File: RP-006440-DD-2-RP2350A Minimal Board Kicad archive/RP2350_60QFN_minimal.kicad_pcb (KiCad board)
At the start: 2 copper layers, 52 x 51 mm, 45 parts, among them J1 USB_C_Receptacle_USB2.0_16P, J2 Conn_02x18_Odd_Even, J3 Conn_02x18_Odd_Even, J4 SM03B-SRSS-TB, SW1 SW_Push, SW2 SW_Push, U1 RP2350_60QFN, U2 NCP1117-3.3_SOT223, U3 W25Q128JVS, Y1 ABM8-272-T3

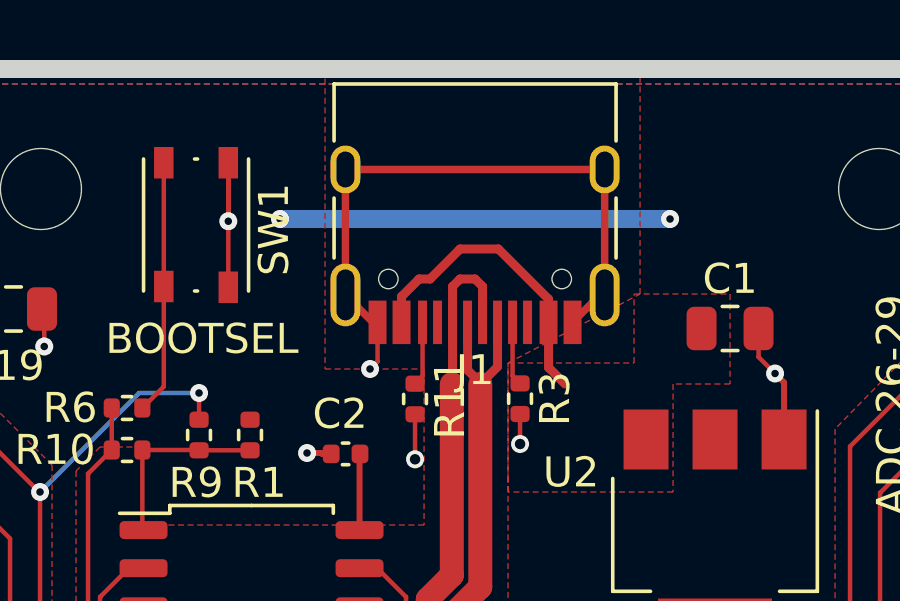
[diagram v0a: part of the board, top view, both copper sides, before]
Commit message: Schematic text
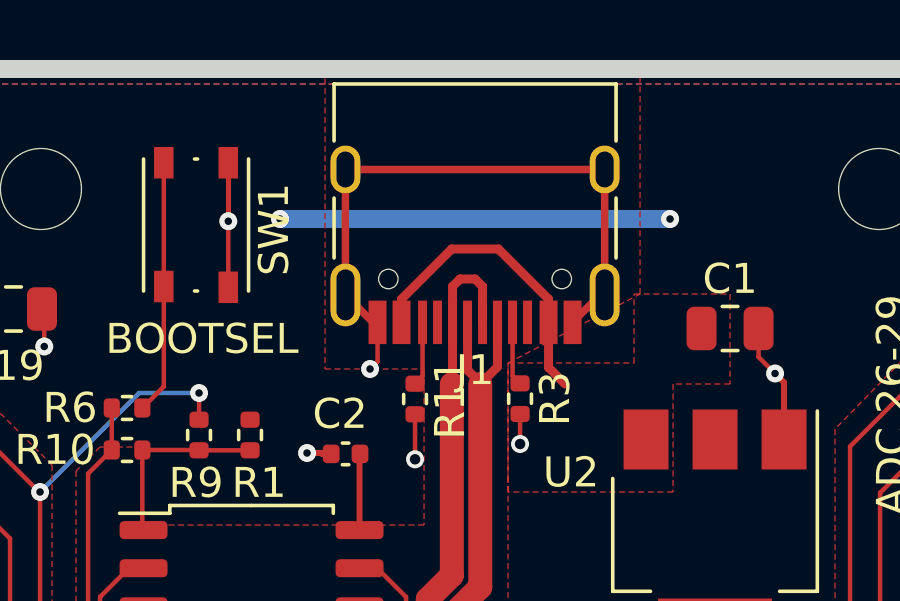
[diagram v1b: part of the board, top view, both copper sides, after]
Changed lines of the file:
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@@
 		(tags "usb usb-c 2.0 pd")
 		(property "Reference" "J1"
-			(at 0 -5.645 360)
+			(at 0 -5.645 0)
 			(layer "F.SilkS")
 			(effects
@@
 		)
 		(property "Value" "USB_C_Receptacle_USB2.0_16P"
-			(at 0 5.1 360)
+			(at 0 5.1 0)
 			(layer "F.Fab")
 			(effects
@@
 		)
 		(fp_text user "${REFERENCE}"
-			(at 0 0 360)
+			(at 0 0 0)
 			(layer "F.Fab")
 			(effects
@@
 	)
 	(segment
-		(start 100 76)
-		(end 101.28 76)
+		(start 102.95 79.95)
+		(end 103.5 80.5)
 		(width 0.3)
 		(layer "F.Cu")
@@
 	)
 	(segment
-		(start 98.05 78.445)
-		(end 98.05 77.585305)
-		(width 0.3)
-		(layer "F.Cu")
-		(net 2)
-	)
-	(segment
-		(start 102.95 79.95)
-		(end 103.5 80.5)
-		(width 0.3)
-		(layer "F.Cu")
-		(net 2)
-	)
-	(segment
-		(start 99 77)
-		(end 100 76)
+		(start 99.72 76)
+		(end 101.28 76)
 		(width 0.3)
 		(layer "F.Cu")
@@
 	)
 	(segment
-		(start 98.635305 77)
-		(end 99 77)
+		(start 102.95 78.445)
+		(end 102.95 79.95)
 		(width 0.3)
 		(layer "F.Cu")
@@
 	)
 	(segment
-		(start 102.95 78.445)
-		(end 102.95 79.95)
+		(start 101.28 76)
+		(end 102.95 77.67)
 		(width 0.3)
 		(layer "F.Cu")
@@
 	)
 	(segment
-		(start 101.28 76)
-		(end 102.95 77.67)
+		(start 98.05 78.445)
+		(end 98.05 77.67)
 		(width 0.3)
 		(layer "F.Cu")
@@
 	)
 	(segment
-		(start 98.05 77.585305)
-		(end 98.635305 77)
+		(start 98.05 77.67)
+		(end 99.72 76)
 		(width 0.3)
 		(layer "F.Cu")
